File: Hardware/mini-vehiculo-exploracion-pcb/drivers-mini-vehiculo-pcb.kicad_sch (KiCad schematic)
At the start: 25 parts, among them J1 Conn_01x08_Pin_drv, J2 Conn_01x02_Pin, J3 Conn_01x02_Motor1, J4 Conn_01x02_Motor2, J5 Conn_01x02_Servo, U3 DRV8873HPWPRQ1, U4 DRV8873HPWPRQ1

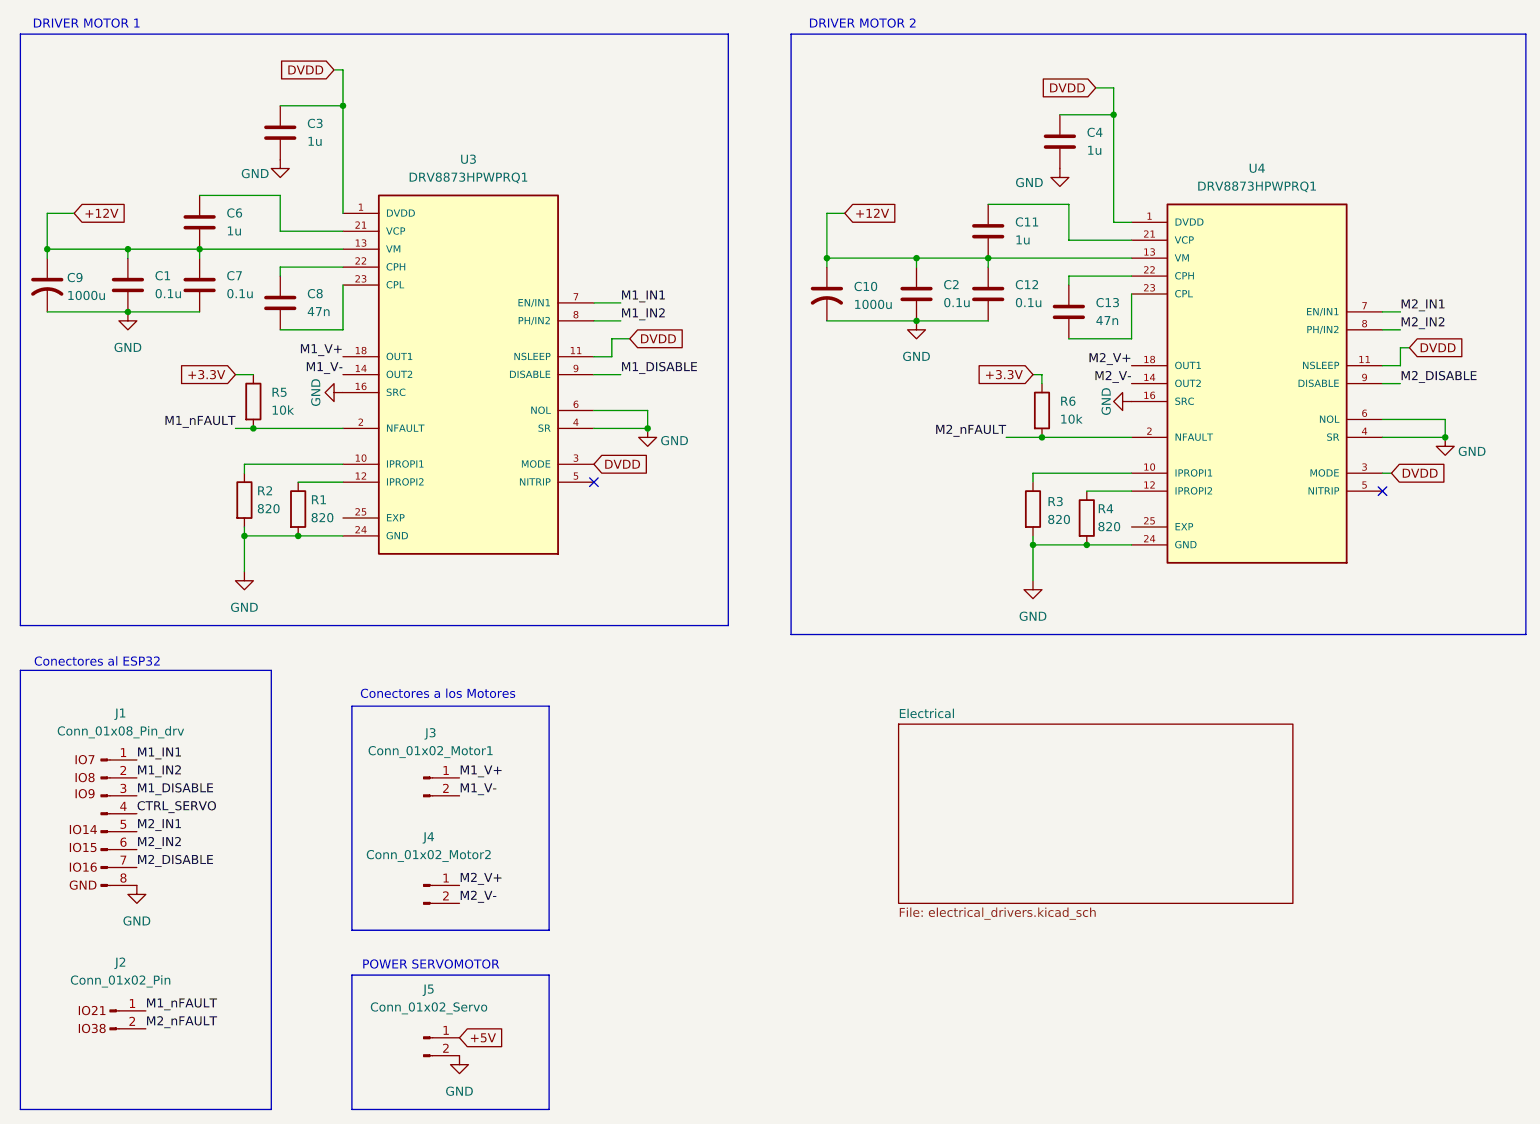
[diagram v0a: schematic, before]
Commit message: updated pcb drv
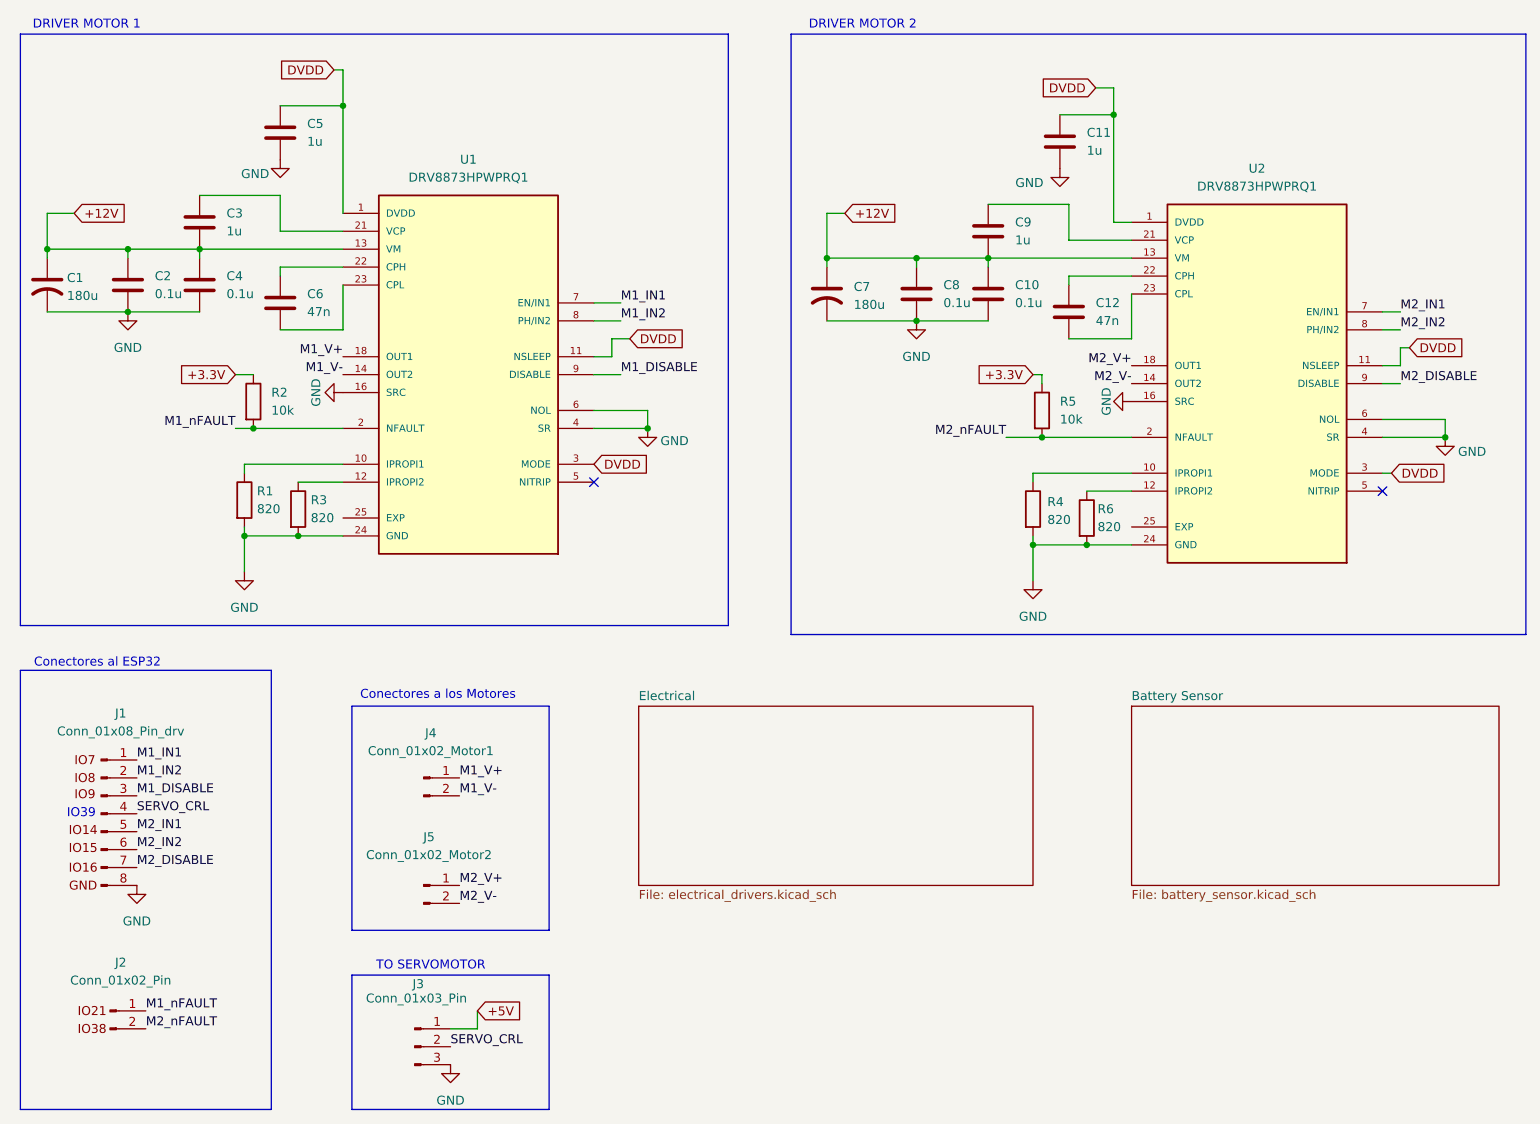
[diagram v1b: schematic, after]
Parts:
- removed J5: Conn_01x02_Servo, symbol Connector:Conn_01x02_Pin
- added J3: Conn_01x03_Pin, symbol Connector:Conn_01x03_Pin
- C1: renamed from C9; value 1000u -> 180u; footprint (none) -> EMZR160ARA221MF61G:CAPAE660X610N
- C7: renamed from C10; value 1000u -> 180u; footprint (none) -> EMZR160ARA221MF61G:CAPAE660X610N
- J1: footprint (none) -> JST_Connectors:JST_8PIN
- renumbered C12 to C10, C4 to C11, C13 to C12, C1 to C2, C6 to C3, C7 to C4, C3 to C5, C8 to C6, C2 to C8, C11 to C9, J3 to J4, J4 to J5, R2 to R1, R5 to R2, R1 to R3, R3 to R4, R6 to R5, R4 to R6, U3 to U1, U4 to U2
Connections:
- net +5V: now also J3.1 (Pin_1)
- net GND: now also J3.3 (Pin_3)
- net CTRL_SERVO renamed SERVO_CRL
- net SERVO_CRL: now also J3.2 (Pin_2)
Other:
- added sheet Battery Sensor (battery_sensor.kicad_sch)
- note added: "IO39"
- note added: "TO SERVOMOTOR"
- note removed: "POWER SERVOMOTOR"
